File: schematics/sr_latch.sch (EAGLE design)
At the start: 1 part, among them IC1 74ALS02D

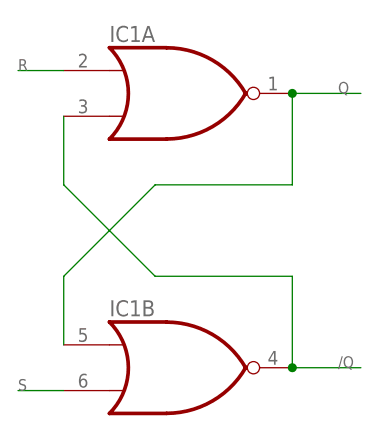
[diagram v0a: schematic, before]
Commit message: Numerous errata
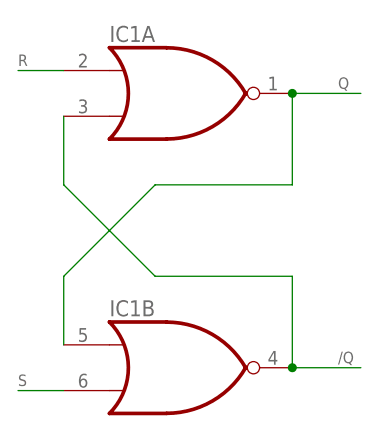
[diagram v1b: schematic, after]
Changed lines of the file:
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@@
 <wire x1="12.7" y1="7.62" x2="12.7" y2="17.78" width="0.1524" layer="91"/>
 <junction x="12.7" y="17.78"/>
-<label x="17.78" y="17.78" size="1.27" layer="95"/>
+<label x="17.78" y="18.288" size="1.27" layer="95"/>
 </segment>
 </net>
@@
 <wire x1="12.7" y1="-2.54" x2="12.7" y2="-12.7" width="0.1524" layer="91"/>
 <junction x="12.7" y="-12.7"/>
-<label x="17.78" y="-12.7" size="1.27" layer="95"/>
+<label x="17.78" y="-12.192" size="1.27" layer="95"/>
 </segment>
 </net>
@@
 <pinref part="IC1" gate="A" pin="I0"/>
 <wire x1="-12.7" y1="20.32" x2="-17.78" y2="20.32" width="0.1524" layer="91"/>
-<label x="-17.78" y="20.32" size="1.27" layer="95"/>
+<label x="-17.78" y="20.828" size="1.27" layer="95"/>
 </segment>
 </net>
@@
 <pinref part="IC1" gate="B" pin="I1"/>
 <wire x1="-12.7" y1="-15.24" x2="-17.78" y2="-15.24" width="0.1524" layer="91"/>
-<label x="-17.78" y="-15.24" size="1.27" layer="95"/>
+<label x="-17.78" y="-14.732" size="1.27" layer="95"/>
 </segment>
 </net>
